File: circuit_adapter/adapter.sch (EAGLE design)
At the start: 12 parts, among them CN1 5035521020, CN3 5035521020, X1 2510-

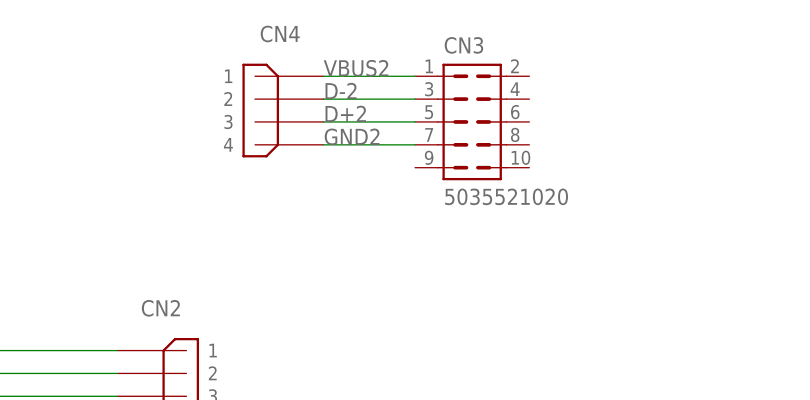
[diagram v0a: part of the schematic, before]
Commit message: Modified adapter circuit and added garber zip
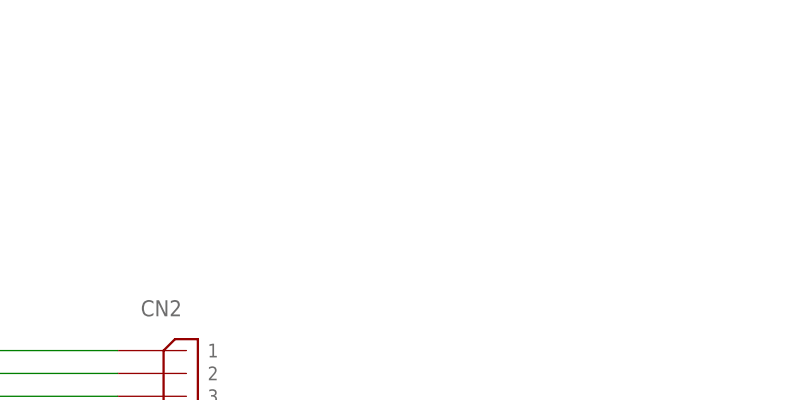
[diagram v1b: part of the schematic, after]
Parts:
- removed CN3: 5035521020, connector:5035521020
- removed CN4: (no value), connector:USB
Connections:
- removed net D+2: CN3.5, CN4.3
- removed net D-2: CN3.3, CN4.2
- removed net GND2: CN3.7, CN4.4
- removed net VBUS2: CN3.1, CN4.1
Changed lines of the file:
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@@
 <?xml version="1.0" encoding="utf-8"?>
 <!DOCTYPE eagle SYSTEM "eagle.dtd">
-<eagle version="9.1.3">
+<eagle version="9.2.0">
 <drawing>
 <settings>
@@
 <part name="SUPPLY4" library="supply2" library_urn="urn:adsk.eagle:library:372" deviceset="DGND" device=""/>
 <part name="SUPPLY5" library="supply2" library_urn="urn:adsk.eagle:library:372" deviceset="DGND" device=""/>
-<part name="CN4" library="connector" deviceset="USB" device=""/>
-<part name="CN3" library="connector" deviceset="5035521020" device=""/>
 </parts>
 <sheets>
@@
 <instance part="SUPPLY5" gate="G$1" x="93.98" y="2.54">
 <attribute name="VALUE" x="91.313" y="-0.635" size="1.778" layer="96"/>
-</instance>
-<instance part="CN4" gate="G$1" x="53.34" y="124.46" rot="MR0">
-<attribute name="NAME" x="55.88" y="133.35" size="1.778" layer="95" rot="MR0"/>
-<attribute name="VALUE" x="43.18" y="119.38" size="1.778" layer="96" rot="MR90"/>
-</instance>
-<instance part="CN3" gate="G$1" x="73.66" y="124.46">
-<attribute name="NAME" x="71.755" y="132.08" size="1.778" layer="95"/>
-<attribute name="VALUE" x="71.755" y="115.2525" size="1.778" layer="96"/>
 </instance>
 </instances>
@@
 </segment>
 </net>
-<net name="VBUS2" class="0">
-<segment>
-<pinref part="CN4" gate="G$1" pin="1"/>
-<pinref part="CN3" gate="G$1" pin="1"/>
-<wire x1="58.42" y1="129.54" x2="68.58" y2="129.54" width="0.1524" layer="91"/>
-<label x="58.42" y="129.54" size="1.778" layer="95"/>
-</segment>
-</net>
-<net name="D-2" class="1">
-<segment>
-<pinref part="CN4" gate="G$1" pin="2"/>
-<pinref part="CN3" gate="G$1" pin="3"/>
-<wire x1="58.42" y1="127" x2="68.58" y2="127" width="0.1524" layer="91"/>
-<label x="58.42" y="127" size="1.778" layer="95"/>
-</segment>
-</net>
-<net name="D+2" class="0">
-<segment>
-<pinref part="CN4" gate="G$1" pin="3"/>
-<pinref part="CN3" gate="G$1" pin="5"/>
-<wire x1="58.42" y1="124.46" x2="68.58" y2="124.46" width="0.1524" layer="91"/>
-<label x="58.42" y="124.46" size="1.778" layer="95"/>
-</segment>
-</net>
-<net name="GND2" class="0">
-<segment>
-<pinref part="CN4" gate="G$1" pin="4"/>
-<pinref part="CN3" gate="G$1" pin="7"/>
-<wire x1="58.42" y1="121.92" x2="68.58" y2="121.92" width="0.1524" layer="91"/>
-<label x="58.42" y="121.92" size="1.778" layer="95"/>
-</segment>
-</net>
